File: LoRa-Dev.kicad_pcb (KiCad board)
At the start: 2 copper layers, 14 parts, among them J2 Barrel_Jack_MountingPin, U1 RPi Pico, U2 LT1963AEQ

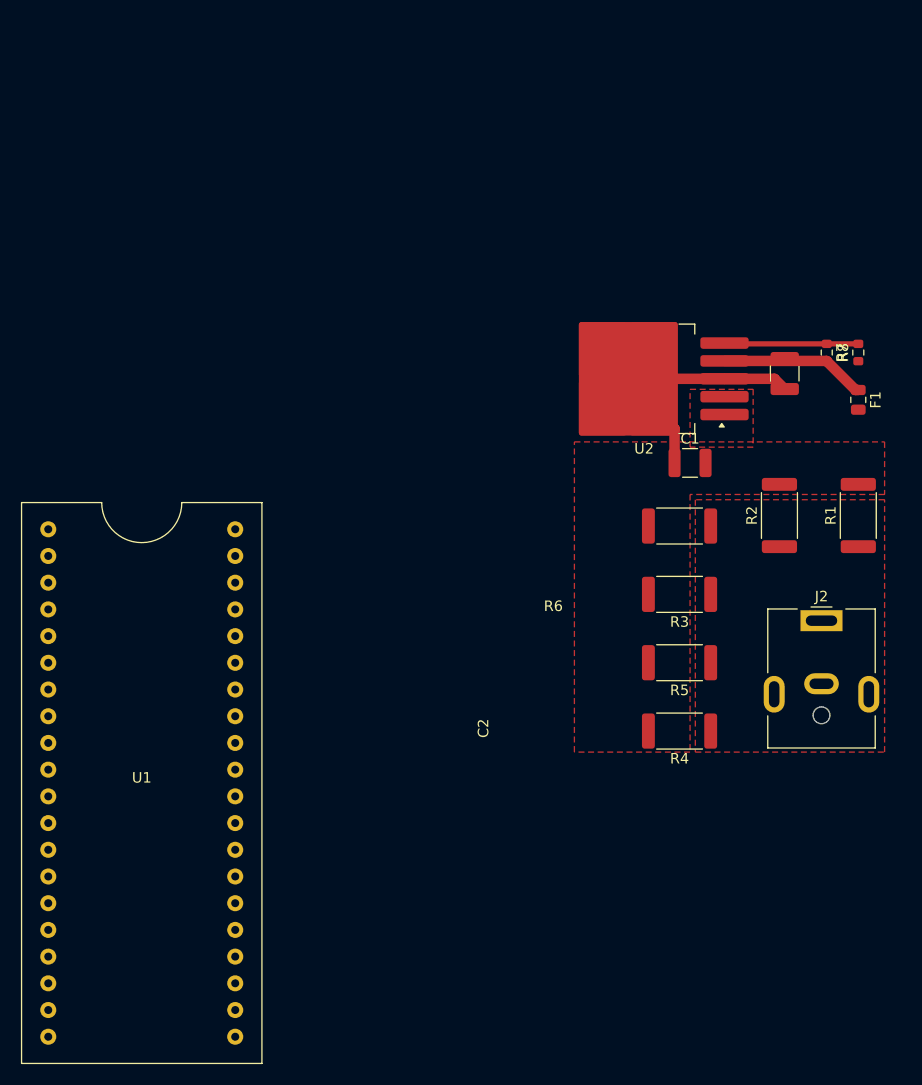
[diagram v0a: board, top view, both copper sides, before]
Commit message: board layout
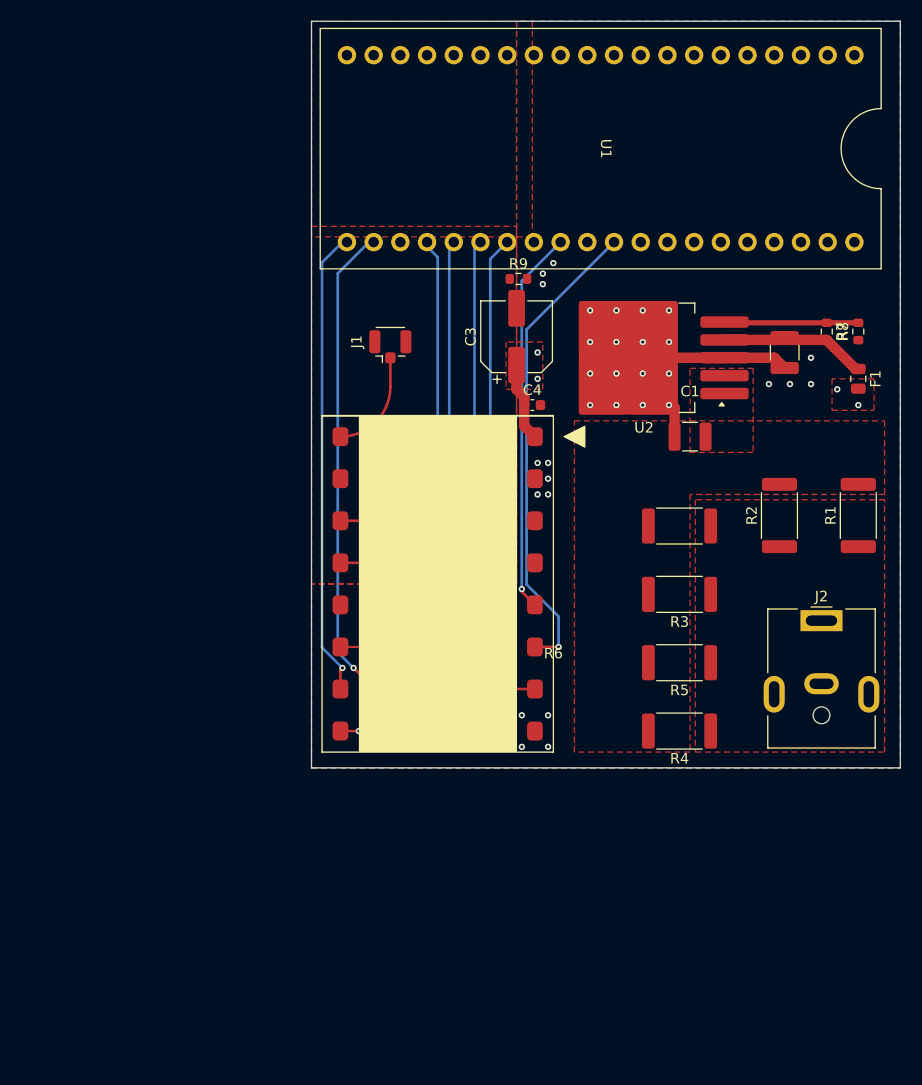
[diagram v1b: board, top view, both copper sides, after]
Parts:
- added C3: 47uF, Capacitor_SMD:CP_Elec_6.3x5.8, F.Cu at (126.5, 59.0)
- added C4: 0.1uF, Capacitor_SMD:C_0603_1608Metric, F.Cu at (128.0, 65.5)
- added J1: Conn_Coaxial_Small, Connector_Coaxial:U.FL_Hirose_U.FL-R-SMT-1_Vertical, F.Cu at (114.5, 60.0)
- added R9: R_Small, Resistor_SMD:R_0603_1608Metric, F.Cu at (126.7, 53.5)
- added U3: LoRa126XF30, LoRa-Dev:LoRa126XF30, F.Cu at (119.0, 82.5)
- moved U1 74.5 mm to (134.5, 41.1), turned to -90 degrees
- moved C1 2.50 mm to (143.0, 68.5)
- moved C2 2.00 mm to (152.0, 60.5)
- moved F1 2.00 mm to (159.0, 63.0)
- moved R7 2.00 mm to (156.0, 58.5)
- moved R8 2.00 mm to (159.0, 58.5)
- moved U2 2.00 mm to (138.6, 61.0)
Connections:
- net Net-(J2-Pad1) renamed /12V
- J2 pad MP: unconnected-(J2-MountPin-PadMP) -> GND
- U1 pad 26: unconnected-(U1-GP20-Pad26) -> /DIO3
- U1 pad 27: unconnected-(U1-GP21-Pad27) -> /DIO1
- U1 pad 29: unconnected-(U1-GP22-Pad29) -> /RESETn
- U1 pad 31: unconnected-(U1-GP26-Pad31) -> /BUSY
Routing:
- net /SPI_CSn: track 0.00 -> 60.4 mm, vias 0 -> 1
- net /SPI_SCK: track 0.00 -> 52.0 mm, vias 0 -> 1
- net RF_VDD: track 0.00 -> 49.8 mm, vias 0 -> 4
- net /BUSY: track 0.00 -> 45.5 mm, vias 0 -> 1
- net /DIO1: track 0.00 -> 45.4 mm, vias 0 -> 1
- net /SPI_MOSI: track 0.00 -> 44.7 mm, vias 0 -> 1
- net /SPI_MISO: track 0.00 -> 44.2 mm, vias 0 -> 1
- net /DIO3: track 0.00 -> 39.5 mm, vias 0 -> 1
- net /RESETn: track 0.00 -> 36.5 mm, vias 0 -> 1
- net /ANT: track 0.00 -> 10.0 mm
- net GND: track 21.3 -> 20.8 mm, vias 0 -> 32
- added copper zone on F.Cu, net /RF_GND
- added copper zone on In1.Cu, net /RF_GND
- added copper zone on B.Cu, net GND
- added copper zone on F.Cu, net GND
- added copper zone on In1.Cu, net GND
- added copper zone on In2.Cu, net GND
- added copper zone on F.Cu, net RF_VDD
- added copper zone on In2.Cu, net RF_VDD
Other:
- board outline added: 56 x 71 mm
- copper layers 2 -> 4

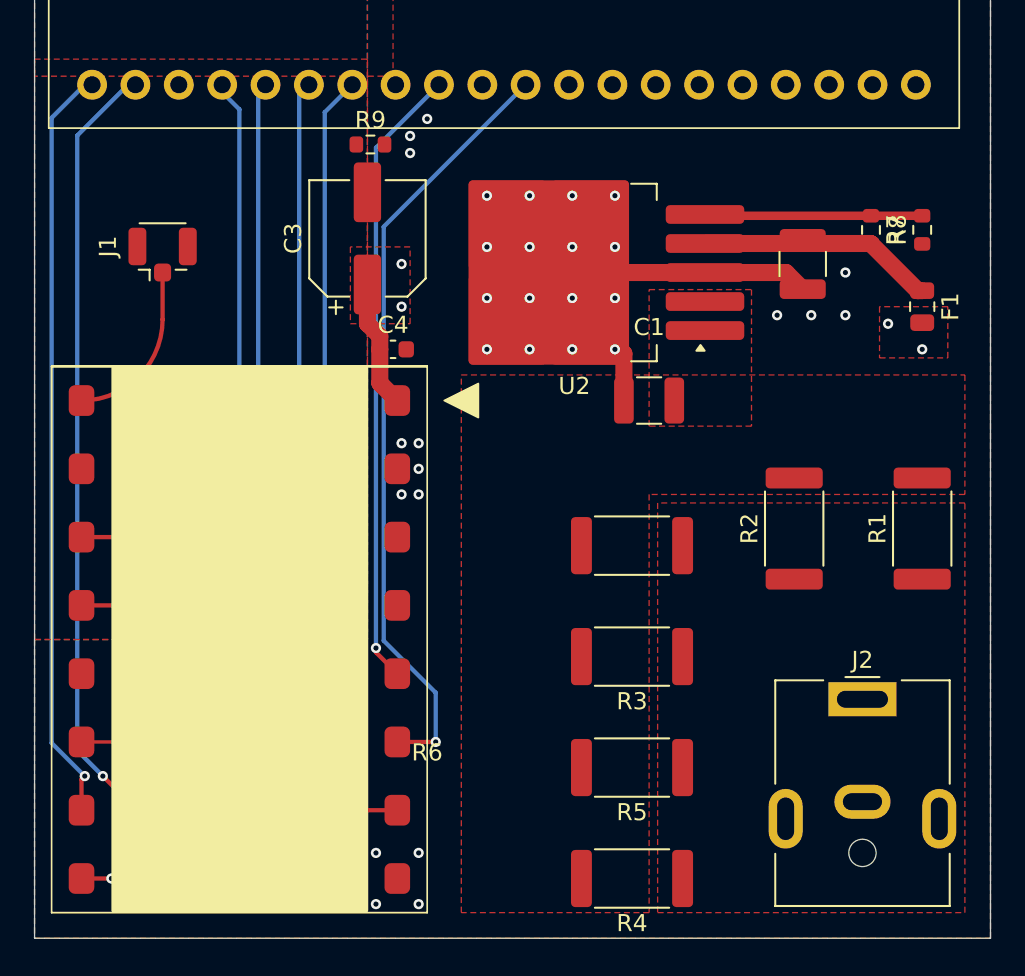
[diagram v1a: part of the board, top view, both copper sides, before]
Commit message: Update silkscreen
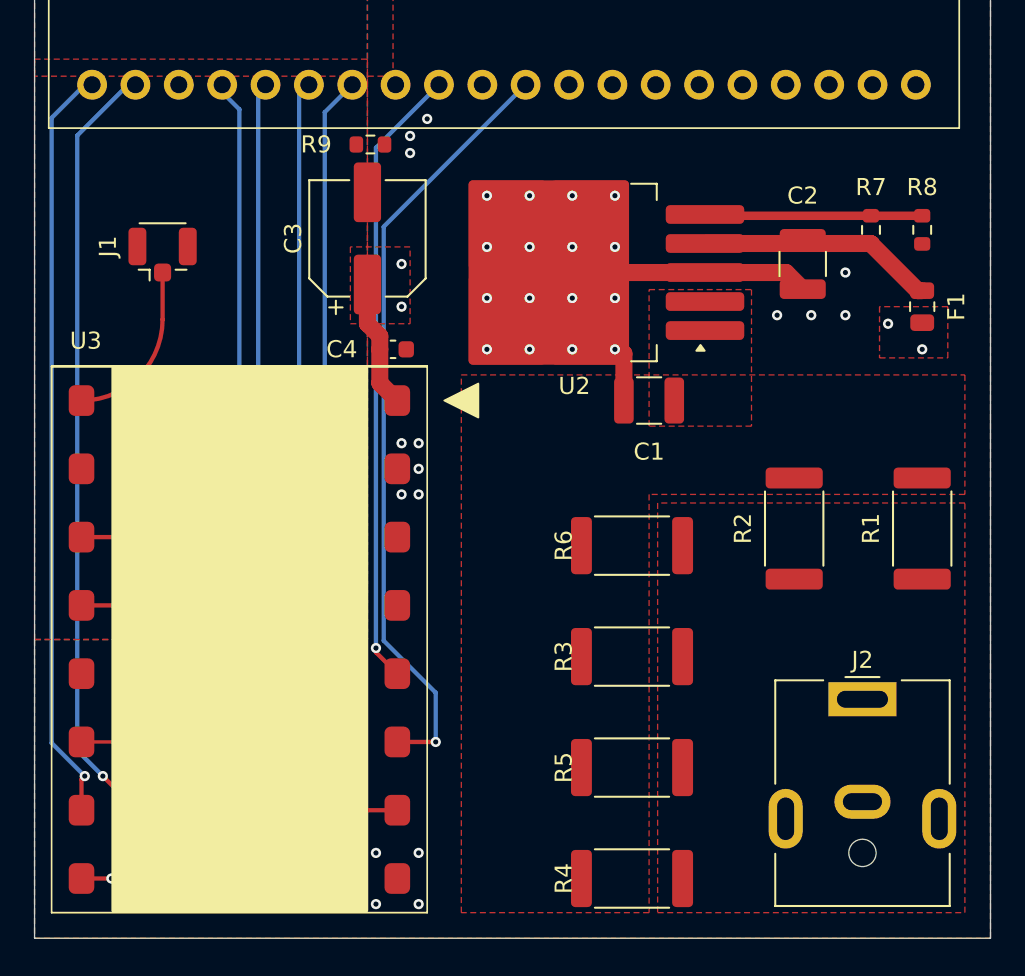
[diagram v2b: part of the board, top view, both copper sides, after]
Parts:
- R7: value 1k5 -> 4k7
- R8: value 4k7 -> 1k5
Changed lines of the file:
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@@
 		(tags "resistor")
 		(property "Reference" "R5"
-			(at 0 -2.62 0)
+			(at 4 0 90)
 			(layer "F.SilkS")
 			(effects
@@
 		(tags "resistor")
 		(property "Reference" "R8"
-			(at 0 -1.43 90)
+			(at 2.5 0 180)
 			(layer "F.SilkS")
 			(effects
@@
 			)
 		)
-		(property "Value" "4k7"
+		(property "Value" "1k5"
 			(at 0 1.43 90)
 			(layer "F.Fab")
@@
 		(tags "resistor")
 		(property "Reference" "R1"
-			(at 0 -2.62 90)
+			(at 0 -3 90)
 			(layer "F.SilkS")
 			(effects
@@
 		(tags "resistor")
 		(property "Reference" "R3"
-			(at 0 -2.62 0)
+			(at 4 0 90)
 			(layer "F.SilkS")
 			(effects
@@
 		(tags "resistor")
 		(property "Reference" "R4"
-			(at 0 -2.62 0)
+			(at 4 0 90)
 			(layer "F.SilkS")
 			(effects
@@
 		)
 		(fp_text user "${REFERENCE}"
-			(at 0.475 0 360)
+			(at 0.475 0 0)
 			(layer "F.Fab")
 			(effects
@@
 		(tags "fuse")
 		(property "Reference" "F1"
-			(at 0 -1.65 90)
+			(at 0 -2 90)
 			(layer "F.SilkS")
 			(effects
@@
 		(at 119 82.5 90)
 		(property "Reference" "U3"
-			(at 2 -0.5 90)
+			(at 17.5 -9 0)
 			(unlocked yes)
 			(layer "F.SilkS")
@@
 		(tags "capacitor")
 		(property "Reference" "C2"
-			(at -33.74 -28.65 90)
+			(at 4 0 180)
 			(layer "F.SilkS")
 			(effects
@@
 		(tags "capacitor")
 		(property "Reference" "C4"
-			(at 0 -1.43 0)
+			(at -3 0 0)
 			(layer "F.SilkS")
 			(effects
@@
 		(tags "capacitor")
 		(property "Reference" "C1"
-			(at 0 -4.3 0)
+			(at 0 3 0)
 			(layer "F.SilkS")
 			(effects
@@
 		(tags "resistor")
 		(property "Reference" "R6"
-			(at 12 -12.12 0)
+			(at 4 0 90)
 			(layer "F.SilkS")
 			(effects
@@
 		(tags "resistor")
 		(property "Reference" "R7"
-			(at 0 -1.43 90)
+			(at -2.5 0 180)
 			(layer "F.SilkS")
 			(effects
@@
 			)
 		)
-		(property "Value" "1k5"
+		(property "Value" "4k7"
 			(at 0 1.43 90)
 			(layer "F.Fab")
@@
 		(tags "resistor")
 		(property "Reference" "R9"
-			(at 0 -1.43 0)
+			(at -3.175 0 0)
 			(layer "F.SilkS")
 			(effects
@@
 		(tags "resistor")
 		(property "Reference" "R2"
-			(at 0 -2.62 90)
+			(at 0 -3 90)
 			(layer "F.SilkS")
 			(effects
